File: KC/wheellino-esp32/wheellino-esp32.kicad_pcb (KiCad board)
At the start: 2 copper layers, 33 parts, among them J1 SR04, J2 Servo, J3 Motor Drivers, J4 Motor Sensors, J5 Contact Sensors, J6 12V, J7 5V, J8 GY521, J9 LCD, U1 3V3

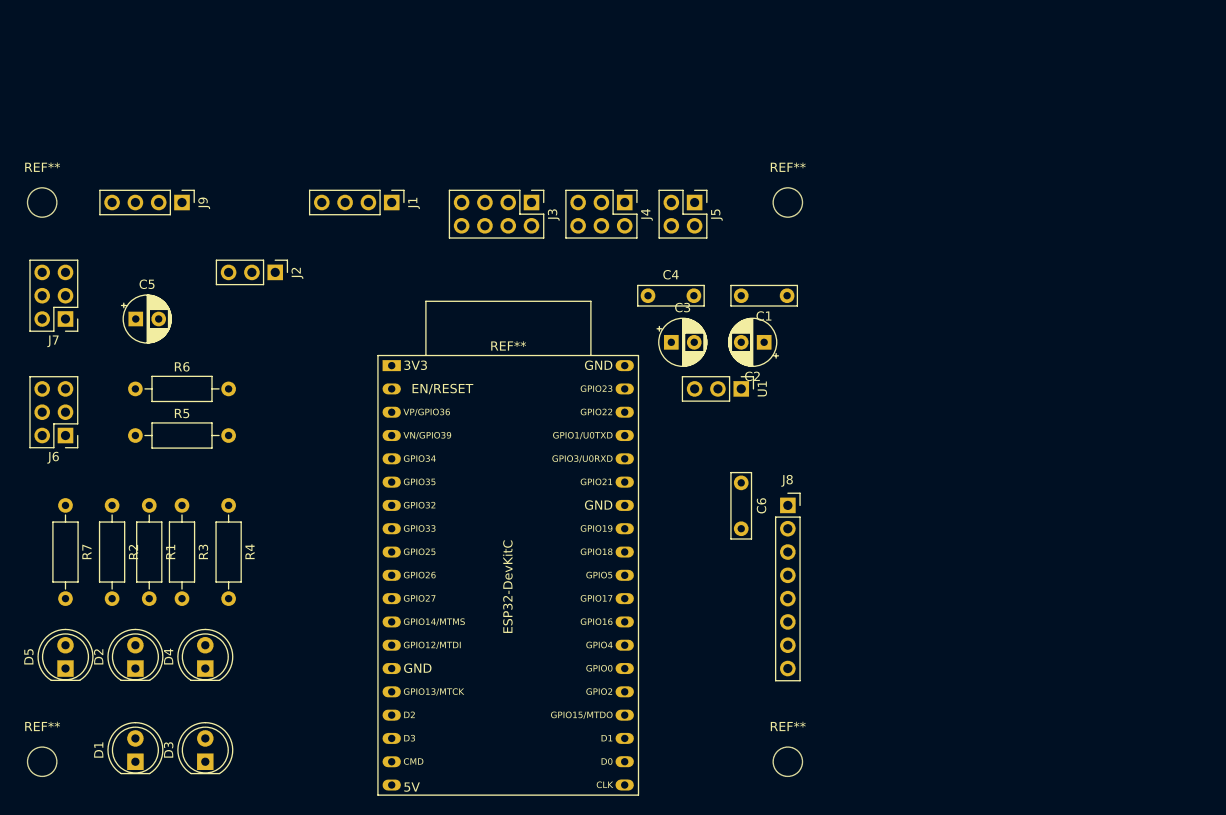
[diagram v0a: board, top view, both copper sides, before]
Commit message: Esp32 board
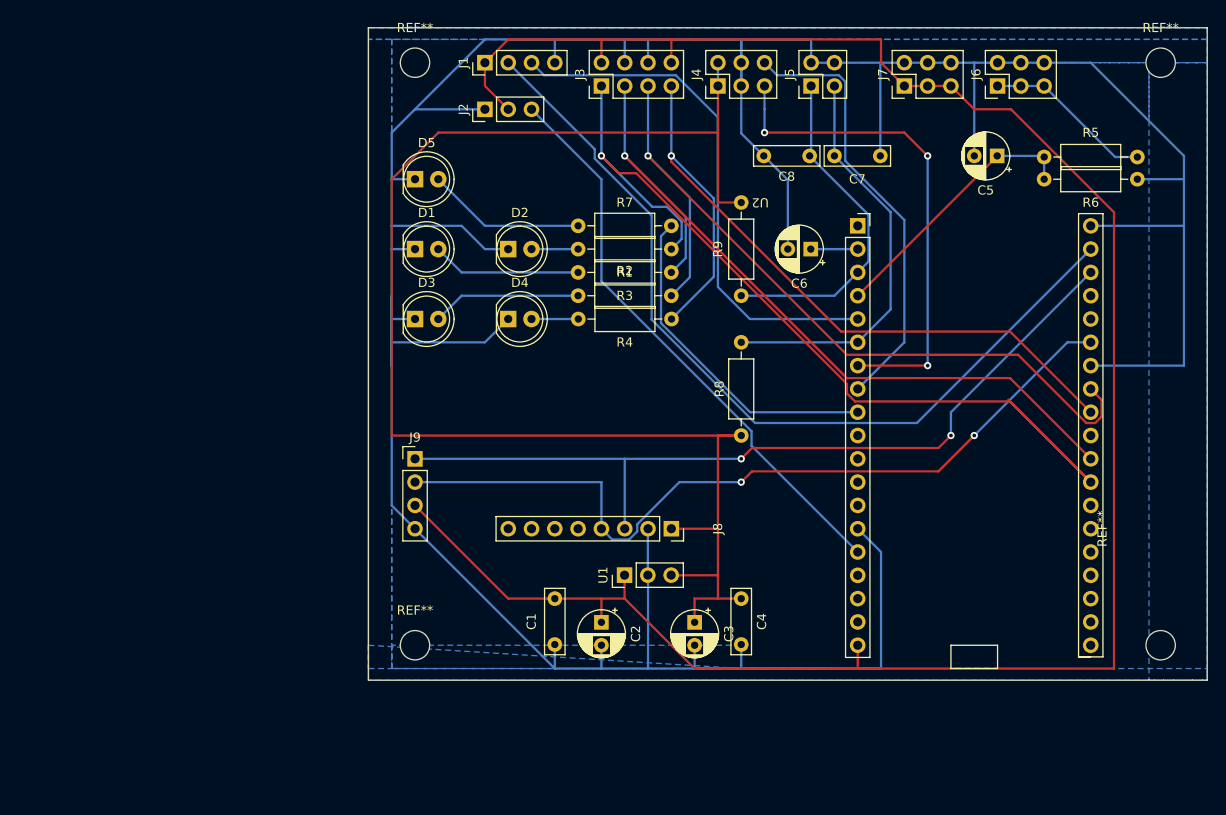
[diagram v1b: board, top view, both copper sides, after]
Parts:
- removed the REF** at (124.5, 83.8)
- added C7: 1n, Capacitor_THT:C_Rect_L7.0mm_W2.0mm_P5.00mm, F.Cu at (172.7, 61.0)
- added C8: 1n, Capacitor_THT:C_Rect_L7.0mm_W2.0mm_P5.00mm, F.Cu at (170.0, 61.0)
- added R8: 10K, Resistor_THT:R_Axial_DIN0207_L6.3mm_D2.5mm_P10.16mm_Horizontal, F.Cu at (162.6, 91.4)
- added R9: 10K, Resistor_THT:R_Axial_DIN0207_L6.3mm_D2.5mm_P10.16mm_Horizontal, F.Cu at (162.6, 66.0)
- added U2: ESP32-DevKitC, Whellino:ESP32, F.Cu at (175.3, 68.6)
- C6: value 1n -> 22uF; footprint Capacitor_THT:C_Rect_L7.0mm_W2.0mm_P5.00mm -> Capacitor_THT:CP_Radial_D5.0mm_P2.50mm
- R1, R2, R3, R4, R7: value 1K -> 220
- R5: value 10K -> 100K
- R6: value 2K -> 22K
- moved R5 113.4 mm to (205.7, 61.1), turned to 180 degrees
- moved J6 108.5 mm to (190.5, 53.3), turned to 90 degrees
- moved R6 101.7 mm to (195.6, 63.5)
- moved C5 95.6 mm to (190.5, 61.0), turned to 180 degrees
- moved J7 94.9 mm to (180.3, 53.3), turned to 90 degrees
- moved R7 72.7 mm to (154.9, 68.6), turned to 180 degrees
- moved R2 67.1 mm to (154.9, 71.1), turned to 180 degrees
- moved D5 65.5 mm to (127.0, 63.5), turned to 0 degrees
- moved D1 63.7 mm to (127.0, 71.1), turned to 0 degrees
- moved R1 62.3 mm to (154.9, 73.7), turned to 180 degrees
- moved D2 61.2 mm to (137.2, 71.1), turned to 0 degrees
- moved R3 58.0 mm to (154.9, 76.2), turned to 180 degrees
- moved D3 53.4 mm to (127.0, 78.7), turned to 0 degrees
- moved R4 52.4 mm to (155.0, 78.7), turned to 180 degrees
- moved D4 50.4 mm to (137.2, 78.7), turned to 0 degrees
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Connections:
- C6 pad 1: +3V3 -> Net-(U2-CHIP_PU)
- J1 pad 1: unconnected-(J1-Pin_1-Pad1) -> +5VD
- J1 pad 2: unconnected-(J1-Pin_2-Pad2) -> Net-(J1-Pin_2)
- J1 pad 3: unconnected-(J1-Pin_3-Pad3) -> Net-(J1-Pin_3)
- J1 pad 4: unconnected-(J1-Pin_4-Pad4) -> GND
- J2 pad 1: unconnected-(J2-Pin_1-Pad1) -> GND
- J2 pad 2: unconnected-(J2-Pin_2-Pad2) -> +5VD
- J2 pad 3: unconnected-(J2-Pin_3-Pad3) -> Net-(J2-Pin_3)
- J3 pad 1: unconnected-(J3-Pin_1-Pad1) -> Net-(J3-Pin_1)
- J3 pad 2: unconnected-(J3-Pin_2-Pad2) -> +5VD
- J3 pad 3: unconnected-(J3-Pin_3-Pad3) -> Net-(J3-Pin_3)
- J3 pad 4: unconnected-(J3-Pin_4-Pad4) -> GND
- J3 pad 5: unconnected-(J3-Pin_5-Pad5) -> Net-(J3-Pin_5)
- J3 pad 6: unconnected-(J3-Pin_6-Pad6) -> GND
- J3 pad 7: unconnected-(J3-Pin_7-Pad7) -> Net-(J3-Pin_7)
- J3 pad 8: unconnected-(J3-Pin_8-Pad8) -> +5VD
- J4 pad 1: unconnected-(J4-Pin_1-Pad1) -> +3V3
- J4 pad 2: unconnected-(J4-Pin_2-Pad2) -> +3V3
- J4 pad 3: unconnected-(J4-Pin_3-Pad3) -> GND
- J4 pad 4: unconnected-(J4-Pin_4-Pad4) -> GND
- J4 pad 5: unconnected-(J4-Pin_5-Pad5) -> Net-(J4-Pin_5)
- J4 pad 6: unconnected-(J4-Pin_6-Pad6) -> Net-(J4-Pin_6)
- J5 pad 1: unconnected-(J5-Pin_1-Pad1) -> Net-(J5-Pin_1)
- J5 pad 2: unconnected-(J5-Pin_2-Pad2) -> GND
- J5 pad 3: unconnected-(J5-Pin_3-Pad3) -> Net-(J5-Pin_3)
- J5 pad 4: unconnected-(J5-Pin_4-Pad4) -> GND
- J8 pad 3: unconnected-(J8-Pin_3-Pad3) -> Net-(J8-Pin_3)
- J8 pad 4: unconnected-(J8-Pin_4-Pad4) -> Net-(J8-Pin_4)
- J9 pad 1: unconnected-(J9-Pin_1-Pad1) -> Net-(J8-Pin_3)
- J9 pad 2: unconnected-(J9-Pin_2-Pad2) -> Net-(J8-Pin_4)
- J9 pad 3: unconnected-(J9-Pin_3-Pad3) -> +5VD
- J9 pad 4: unconnected-(J9-Pin_4-Pad4) -> GND
- R1 pad 1: unconnected-(R1-Pad1) -> Net-(J3-Pin_3)
- R2 pad 1: unconnected-(R2-Pad1) -> Net-(J3-Pin_1)
- R3 pad 1: unconnected-(R3-Pad1) -> Net-(J3-Pin_5)
- R4 pad 1: unconnected-(R4-Pad1) -> Net-(J3-Pin_7)
- R7 pad 1: unconnected-(R7-Pad1) -> Net-(U2-DAC_1/ADC2_CH8/GPIO25)
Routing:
- net GND: track 0.00 -> 399.6 mm
- net +5VD: track 0.00 -> 233.7 mm
- net +3V3: track 0.00 -> 159.7 mm
- net Net-(J3-Pin_1): track 0.00 -> 104.2 mm, vias 0 -> 1
- net Net-(J1-Pin_2): track 0.00 -> 94.9 mm
- net Net-(J8-Pin_3): track 0.00 -> 91.2 mm, vias 0 -> 2
- net Net-(J3-Pin_5): track 0.00 -> 90.9 mm, vias 0 -> 1
- net Net-(J8-Pin_4): track 0.00 -> 88.6 mm, vias 0 -> 2
- net Net-(J3-Pin_3): track 0.00 -> 88.2 mm, vias 0 -> 1
- net Net-(J3-Pin_7): track 0.00 -> 86.9 mm, vias 0 -> 1
- net Net-(J2-Pin_3): track 0.00 -> 63.0 mm
- net Net-(J1-Pin_3): track 0.00 -> 58.0 mm
- net Net-(J4-Pin_5): track 0.00 -> 54.4 mm, vias 0 -> 3
- net Net-(J4-Pin_6): track 0.00 -> 47.9 mm
- net Net-(J5-Pin_3): track 0.00 -> 44.7 mm
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- added copper zone on B.Cu, net GND
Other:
- board outline added: 91.4 x 71.1 mm
